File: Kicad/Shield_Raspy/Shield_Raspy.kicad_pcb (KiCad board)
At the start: 2 copper layers, 104.1 x 91.4 mm, 4 parts, among them J1 Raspberry_Pi_2_3, K1 HEADER_FEMALE_5x2_1.27mm_SMD, U1 CO2, U2 NUCLEO-L432KC

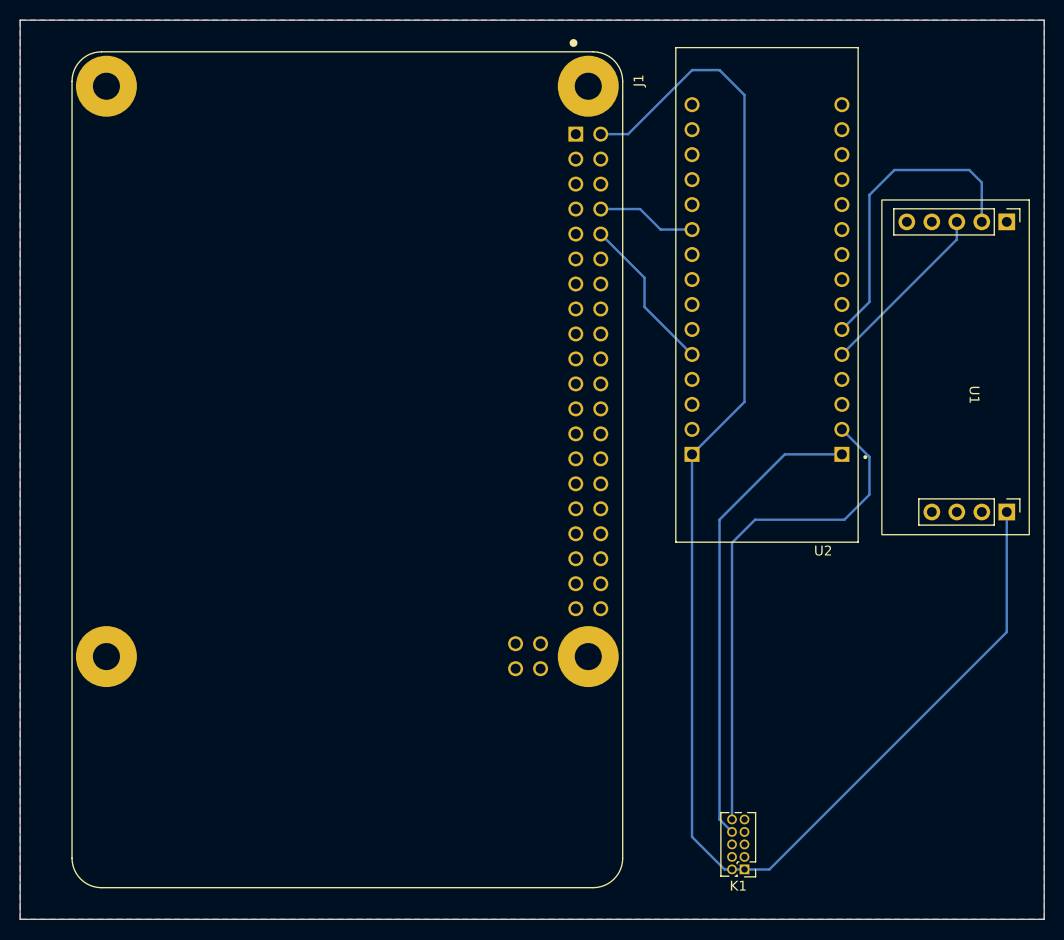
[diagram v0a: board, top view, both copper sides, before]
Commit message: Add files via upload
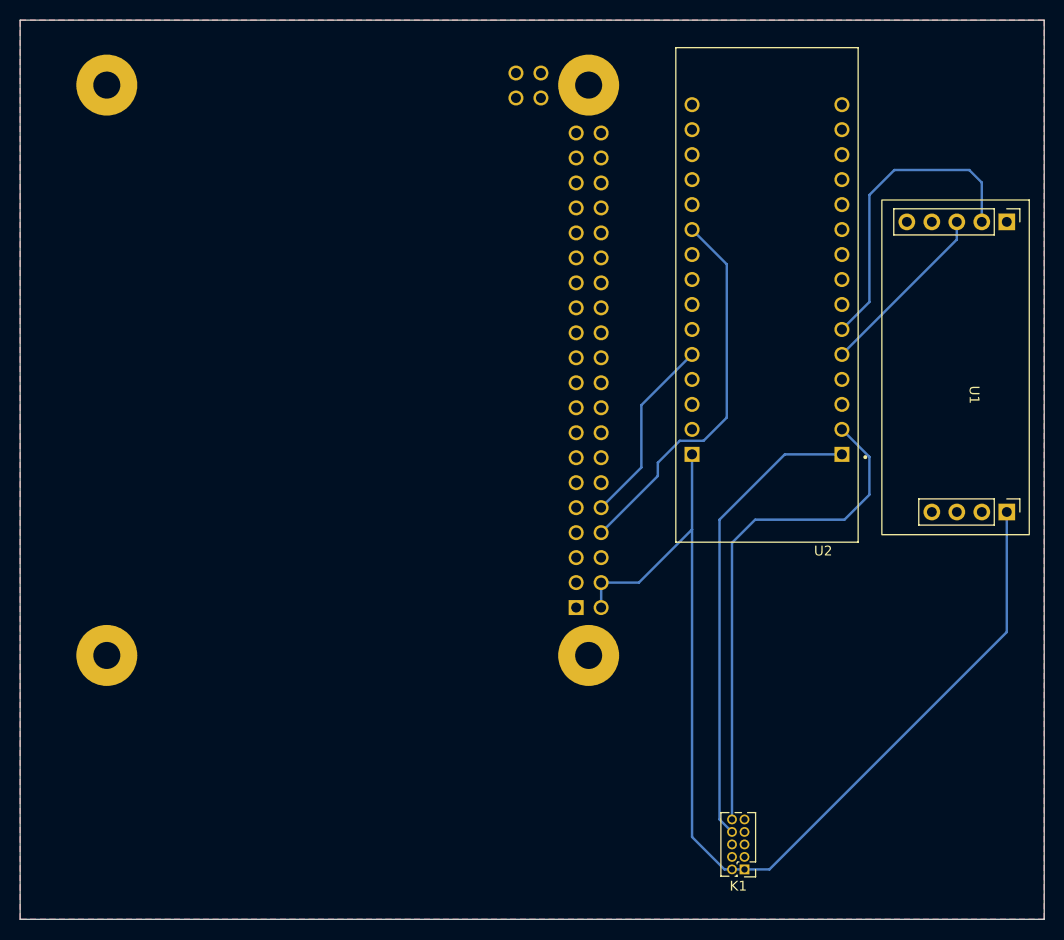
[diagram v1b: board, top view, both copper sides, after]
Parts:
- J1: moved to B.Cu
- moved J1 20.1 mm to (129.8, 68.8), turned to 90 degrees
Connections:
- J1 pad 14: unconnected-(J1-Pad14) -> GND
- J1 pad 20: unconnected-(J1-Pad20) -> GND
- J1 pad 25: unconnected-(J1-Pad25) -> GND
- J1 pad 30: unconnected-(J1-Pad30) -> GND
- J1 pad 34: unconnected-(J1-Pad34) -> GND
- J1 pad 39: unconnected-(J1-Pad39) -> GND
- J1 pad 4: unconnected-(J1-Pad4) -> +5V
- J1 pad 9: unconnected-(J1-Pad9) -> GND
- U2 pad CN3_4: unconnected-(U2-PadCN3_4) -> GND
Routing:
- net +5V: track 151.6 -> 108.5 mm
- net UART_Nucleo_RX_RPi_TX: track 10.1 -> 39.0 mm
- net UART_Nucleo_TX_RPi_RX: track 16.1 -> 19.4 mm
